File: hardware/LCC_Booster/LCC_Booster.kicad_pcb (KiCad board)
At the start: 2 copper layers, 90 x 100 mm, 84 parts, among them J1 Screw_Terminal_01x08, J2 54-00166, J3 RJHSE508002, SW1 SW_Push, U1 SN74HC253DR, U10 MCP2562-E-SN, U11 6N137, U12 6N137, U2 DRV8874PWPR, U3 SN74HC253DR, U4 DRV8874PWPR, U5 SN74HC253DR, U6 DRV8874PWPR, U7 SN74HC253DR, U8 DRV8874PWPR, U9 MCP2518FD-xQBB, Y1 ECS-400-20-46X

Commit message: Added location holes to solder paste template
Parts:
- H1, H2, H3, H4: footprint MountingHole:MountingHole_4.3mm_M4_Pad_Via -> MountingHoles:MountingHole_4.3mm_M4_Pad_Via_PasteAlign

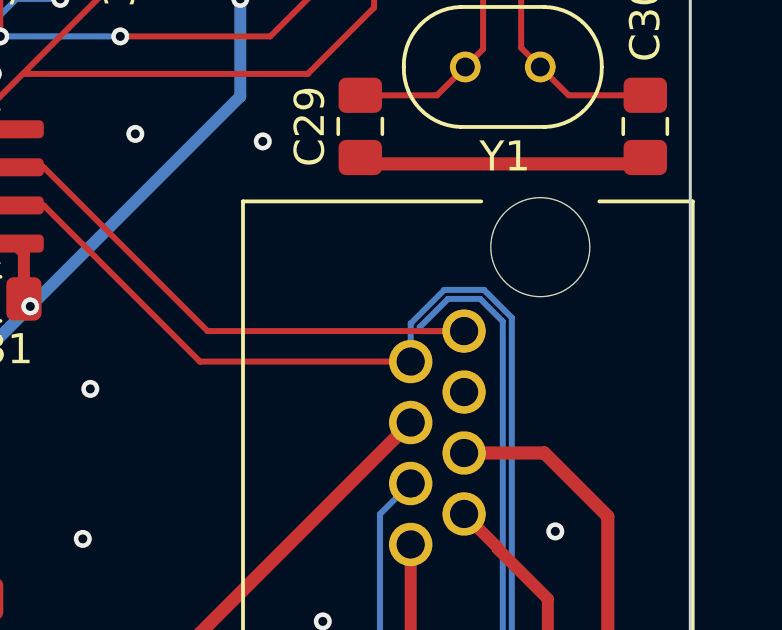
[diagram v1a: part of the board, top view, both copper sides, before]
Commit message: PicoLCC
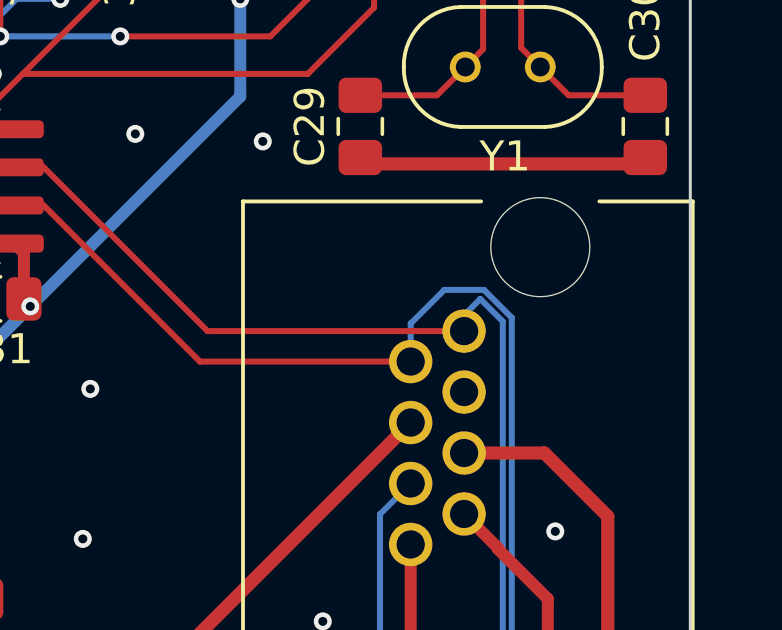
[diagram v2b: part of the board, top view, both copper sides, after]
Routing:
- net /can_h: track 40.3 -> 37.6 mm
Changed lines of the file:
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@@
-	)
-	(segment
-		(start 102.46 93.137)
-		(end 102.612 93.289)
-		(width 0.2)
-		(layer "B.Cu")
-		(net 38)
 	)
 	(segment
@@
 	)
 	(segment
-		(start 101.924264 75.75)
-		(end 100.98 76.694264)
+		(start 103 75.75)
+		(end 102.46 76.29)
 		(width 0.2)
 		(layer "B.Cu")
@@
 	)
 	(segment
-		(start 103 75.75)
-		(end 101.924264 75.75)
+		(start 102.46 93.137)
+		(end 102.612 93.289)
 		(width 0.2)
 		(layer "B.Cu")
@@
 	)
 	(segment
-		(start 100.98 76.803)
-		(end 101 76.823)
-		(width 0.2)
-		(layer "B.Cu")
-		(net 38)
-	)
-	(segment
-		(start 100.98 76.694264)
-		(end 100.98 76.803)
-		(width 0.2)
-		(layer "B.Cu")
-		(net 38)
-	)
-	(segment
-		(start 101 76.823)
+		(start 102.46 76.29)
 		(end 102.46 76.823)
 		(width 0.2)
